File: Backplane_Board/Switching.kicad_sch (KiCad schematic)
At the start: 20 parts, among them J30 Conn_01x02, J31 Conn_01x02, Q3 ZXMN3A14F, Q4 ZXMN3A14F

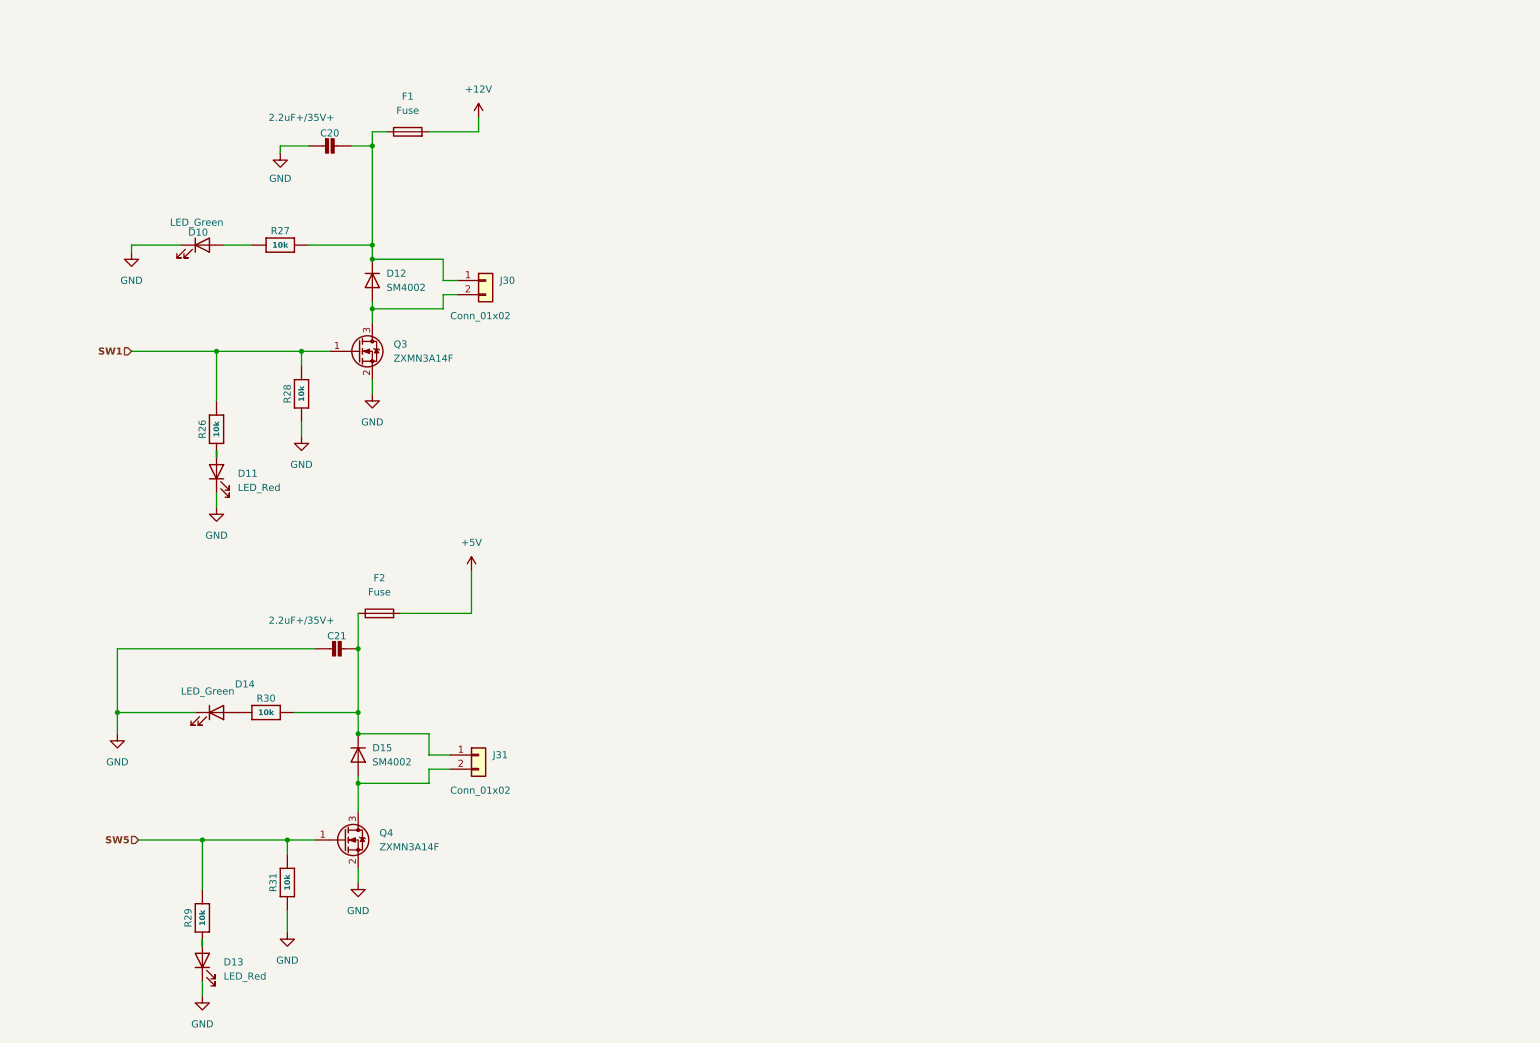
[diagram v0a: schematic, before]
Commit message: ready for final schmatic review
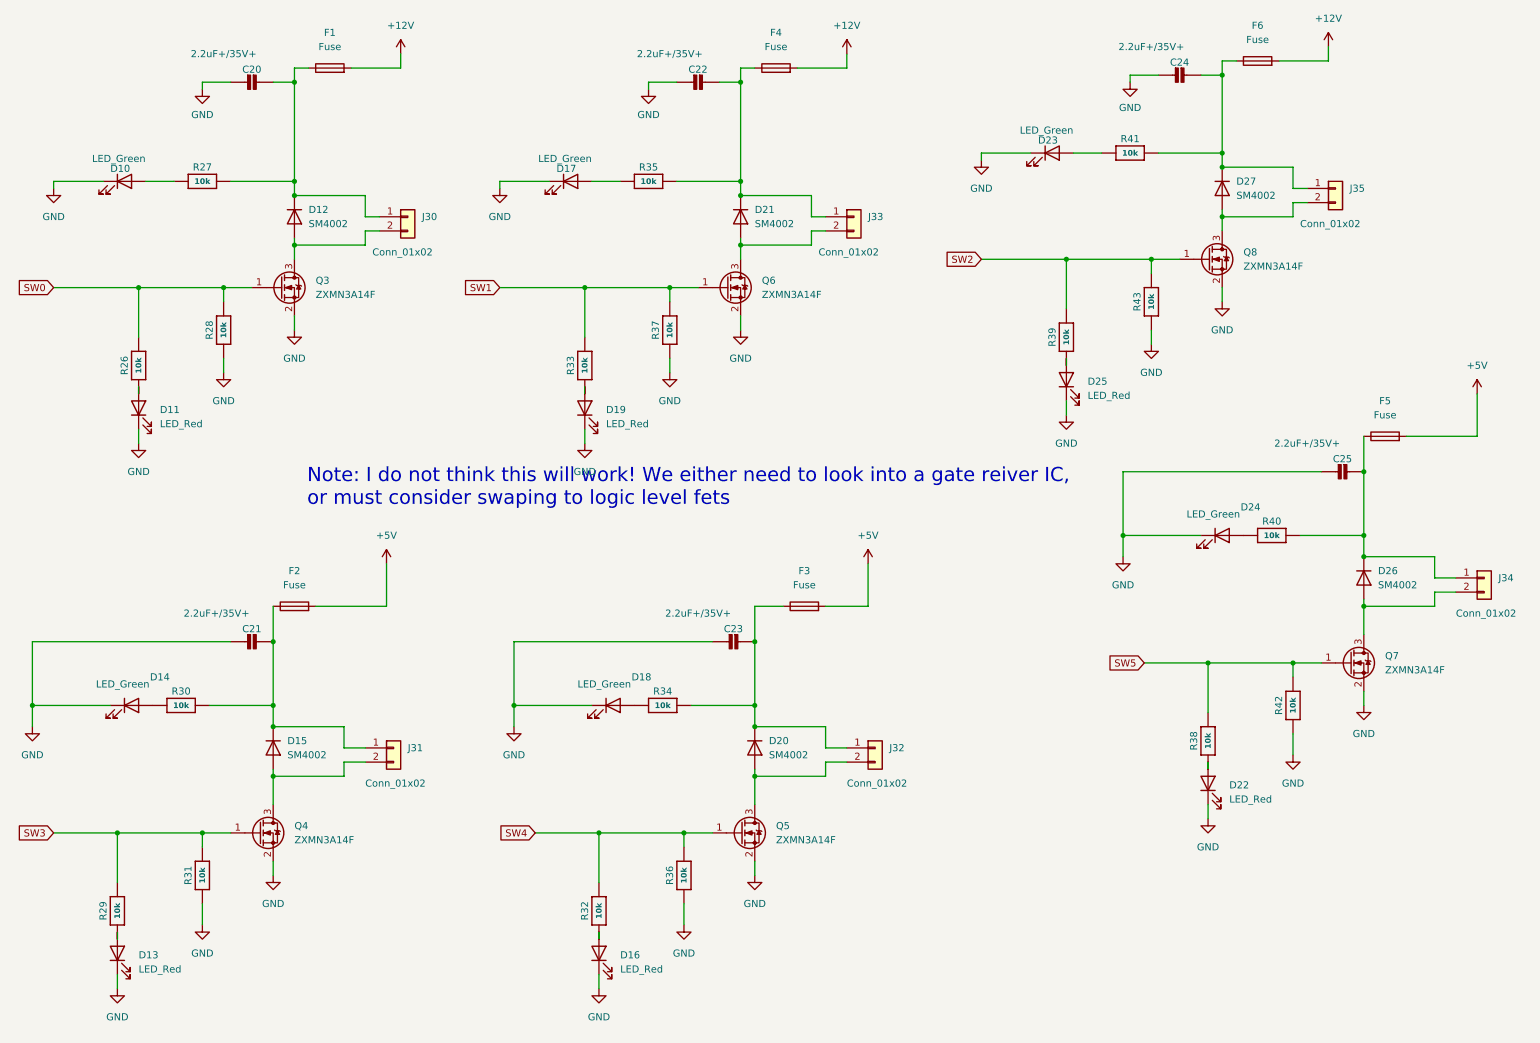
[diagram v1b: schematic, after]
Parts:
- added C22, C23, C24, C25: 2.2uF+/35V+, Capacitor_SMD:C_0805_2012Metric, symbol Adafruit MOSFET Driver STEMMA Breakout-eagle-import:CAP_CERAMIC0805-NOOUTLINE
- added D16, D19, D22, D25: LED_Red, LED_SMD:LED_0603_1608Metric, symbol Device:LED
- added D17, D18, D23, D24: LED_Green, LED_SMD:LED_0603_1608Metric, symbol Device:LED
- added D20, D21, D26, D27: SM4002, Diode_SMD:D_SOD-123F, symbol Diode:SM4002
- added F3, F4, F5, F6: Fuse, Fuse:Fuse_0805_2012Metric, symbol Device:Fuse
- added J32, J33, J34, J35: Conn_01x02, Rpi_Pico_header:Molex_Micro-Latch_53253-0270_1x02_P2.00mm_Vertical_3D_model, symbol Connector_Generic:Conn_01x02
- added Q5, Q6, Q7, Q8: ZXMN3A14F, Package_TO_SOT_SMD:SOT-23, symbol Transistor_FET:ZXMN3A14F
- added R32, R33, R34, R35, R36, R37, R38, R39, R40, R41, R42, R43: 10k, Resistor_SMD:R_0805_2012Metric, symbol Adafruit MOSFET Driver STEMMA Breakout-eagle-import:RESISTOR_0603_NOOUT
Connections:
- net +12V: now also F4.2, F6.2
- net +5V: now also F3.2, F5.2
- net GND: now also C22.2, C23.2, C24.2, C25.2, D16.1 (K), D17.1 (K), D18.1 (K), D19.1 (K), D22.1 (K), D23.1 (K), D24.1 (K), D25.1 (K), Q5.2 (S), Q6.2 (S), Q7.2 (S), Q8.2 (S), R36.1, R37.1, R42.1, R43.1
- net SW1: now also Q6.1 (G), R33.2, R37.2; no longer Q3.1 (G), R26.2, R28.2
- net SW5: now also Q7.1 (G), R38.2, R42.2; no longer Q4.1 (G), R29.2, R31.2
- new net: C25.1, D26.1 (K), F5.1, J34.1 (Pin_1), R40.2
- new net: D24.2 (A), R40.1
- new net: D27.2 (A), J35.2 (Pin_2), Q8.3 (D)
- new net: D16.2 (A), R32.1
- new net: D19.2 (A), R33.1
- new net: D22.2 (A), R38.1
- new net: C22.1, D21.1 (K), F4.1, J33.1 (Pin_1), R35.2
- new net: D21.2 (A), J33.2 (Pin_2), Q6.3 (D)
- new net: D17.2 (A), R35.1
- new net: D26.2 (A), J34.2 (Pin_2), Q7.3 (D)
- new net: D23.2 (A), R41.1
- new net: D25.2 (A), R39.1
- new net: C24.1, D27.1 (K), F6.1, J35.1 (Pin_1), R41.2
- new net: C23.1, D20.1 (K), F3.1, J32.1 (Pin_1), R34.2
- new net: D20.2 (A), J32.2 (Pin_2), Q5.3 (D)
- new net: D18.2 (A), R34.1
- new net SW0: Q3.1 (G), R26.2, R28.2
- new net SW2: Q8.1 (G), R39.2, R43.2
- new net SW3: Q4.1 (G), R29.2, R31.2
- new net SW4: Q5.1 (G), R32.2, R36.2
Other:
- note added: "Note: I do not think this will work! We either need to look into a gate reiver IC, or must consider swaping to logic level fets"
- moved on the sheet: C20, C21, D10, D11, D12, D13, D14, D15, F1, F2, J30, J31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
